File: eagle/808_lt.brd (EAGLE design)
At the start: 100 x 80 mm, 54 parts, among them IC1 TL071P, IC2 TL072P, Q1 2N3904, Q2 2N3906, Q3 2N3904, SW8 MSS42_SW_4PDT

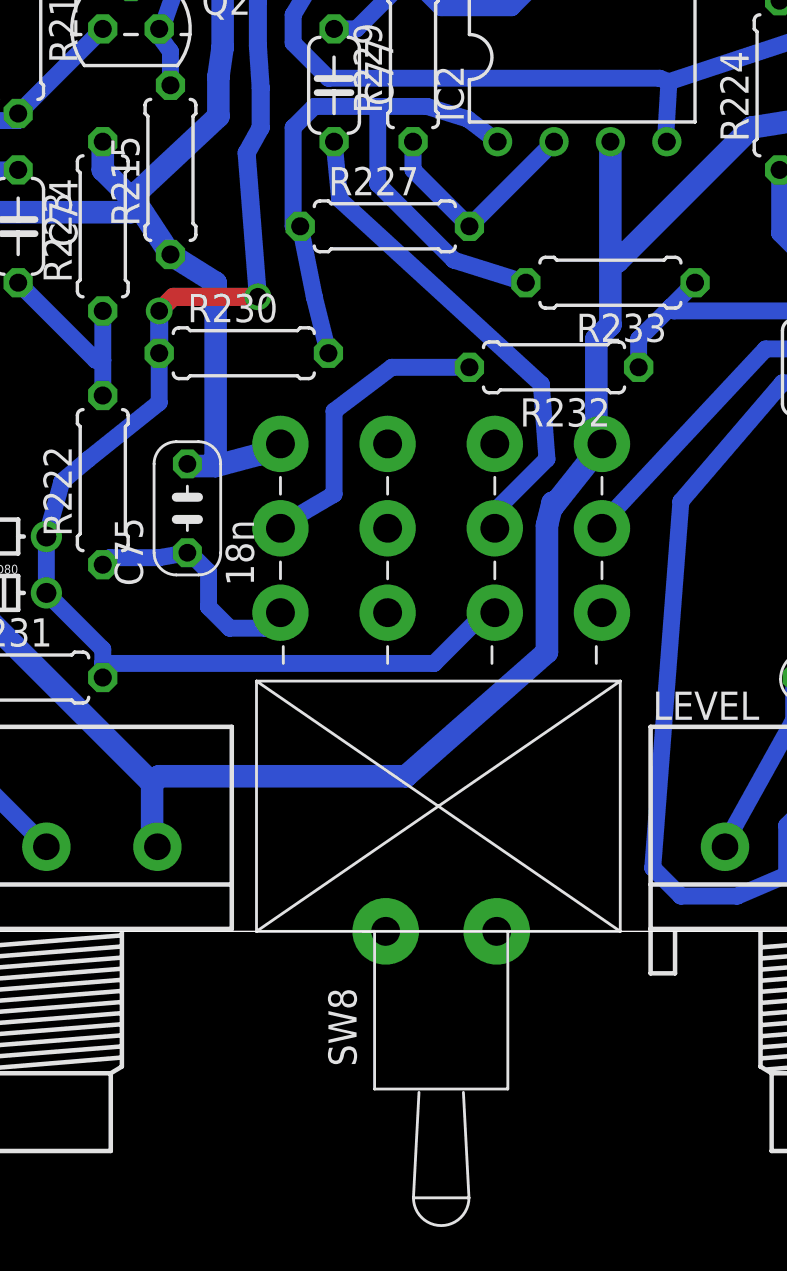
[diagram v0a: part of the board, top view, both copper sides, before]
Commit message: tweaks
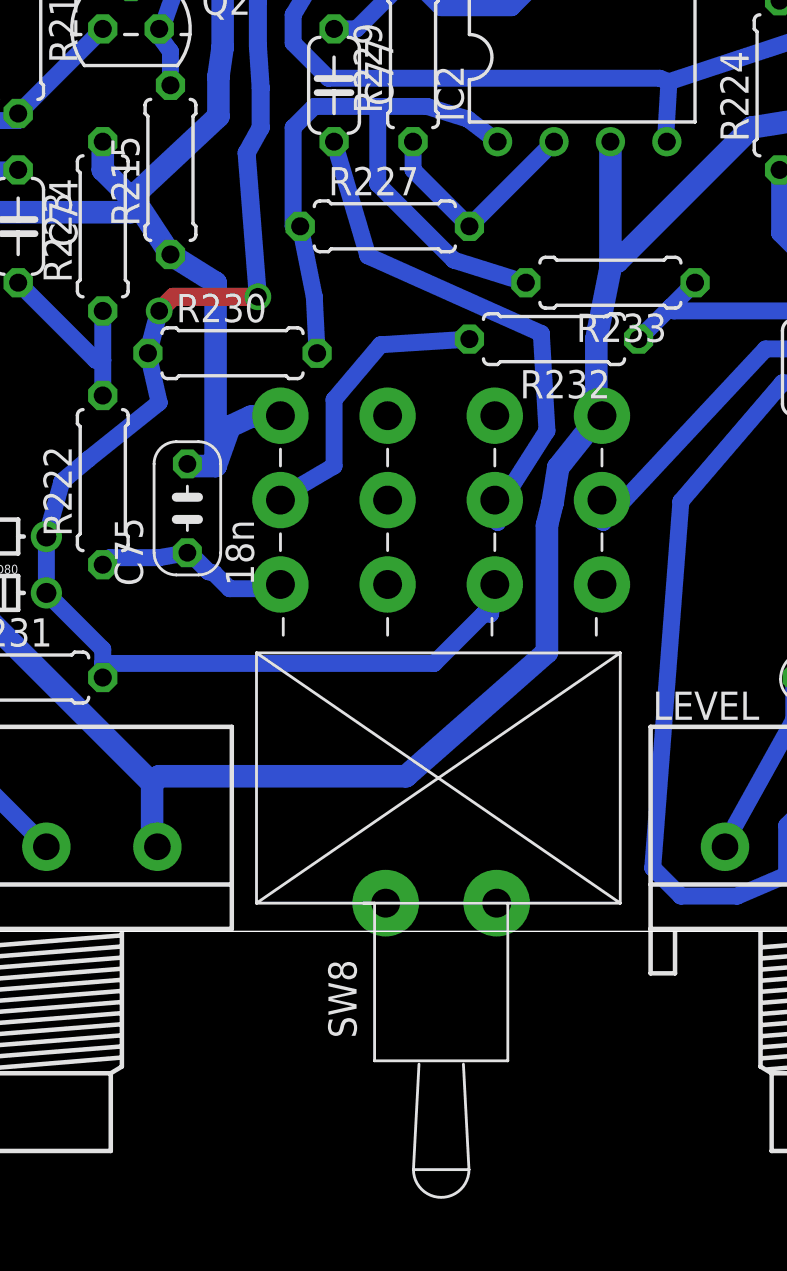
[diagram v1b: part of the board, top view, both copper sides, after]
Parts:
- moved R232 1.27 mm to (57.1, 26.7)
- moved SW8 1.27 mm to (52.1, 1.27)
- moved R230 0.51 mm to (42.7, 26.0)
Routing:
- net N$264: track 10.9 -> 8.96 mm
- net N$271: track 22.4 -> 24.1 mm
- net N$251: track 81.7 -> 83.0 mm
- net N$259: track 11.1 -> 9.85 mm
- net GND: track 423.1 -> 423.9 mm
- net N$111: track 23.3 -> 24.0 mm
